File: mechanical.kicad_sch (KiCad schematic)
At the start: 9 parts

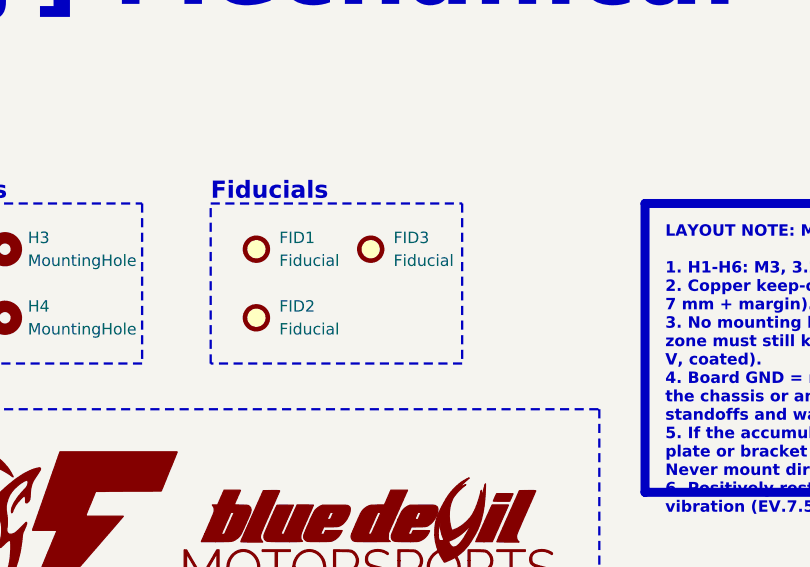
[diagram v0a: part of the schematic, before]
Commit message: PCB&SCH[Fid]: Added 3 fiductals on the back for fab.
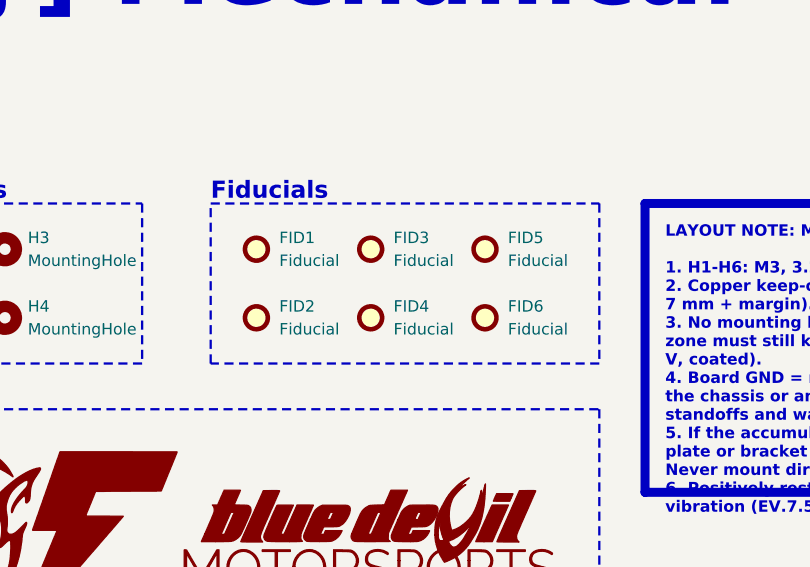
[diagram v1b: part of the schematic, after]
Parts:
- added FID4, FID5, FID6: Fiducial, Fiducial:Fiducial_0.5mm_Mask1mm, symbol Mechanical:Fiducial
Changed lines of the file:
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@@
 	(rectangle
 		(start 147.32 50.8)
-		(end 175.26 68.58)
+		(end 190.5 68.58)
 		(stroke
 			(width 0.254)
@@
 	(symbol
 		(lib_id "Mechanical:Fiducial")
+		(at 165.1 63.5 0)
+		(unit 1)
+		(body_style 1)
+		(exclude_from_sim no)
+		(in_bom no)
+		(on_board yes)
+		(in_pos_files yes)
+		(dnp no)
+		(fields_autoplaced yes)
+		(property "Reference" "FID4"
+			(at 167.64 62.23 0)
+			(show_name no)
+			(do_not_autoplace no)
+			(effects
+				(font
+					(size 1.27 1.27)
+				)
+				(justify left)
+			)
+		)
+		(property "Value" "Fiducial"
+			(at 167.64 64.77 0)
+			(show_name no)
+			(do_not_autoplace no)
+			(effects
+				(font
+					(size 1.27 1.27)
+				)
+				(justify left)
+			)
+		)
+		(property "Footprint" "Fiducial:Fiducial_0.5mm_Mask1mm"
+			(at 165.1 63.5 0)
+			(hide yes)
+			(show_name no)
+			(do_not_autoplace no)
+			(effects
+				(font
+					(size 1.27 1.27)
+				)
+			)
+		)
+		(property "Datasheet" ""
+			(at 165.1 63.5 0)
+			(hide yes)
+			(show_name no)
+			(do_not_autoplace no)
+			(effects
+				(font
+					(size 1.27 1.27)
+				)
+			)
+		)
+		(property "Description" "Fiducial Marker"
+			(at 165.1 63.5 0)
+			(hide yes)
+			(show_name no)
+			(do_not_autoplace no)
+			(effects
+				(font
+					(size 1.27 1.27)
+				)
+			)
+		)
+		(instances
+			(project "bms_slave"
+				(path "/f9e05184-c88b-4a88-ae9c-ab2bdb32be7c/c5103ceb-5325-4a84-a025-9638a412984e/f4a7f626-808e-4d0f-b4d4-b24a2b39d327"
+					(reference "FID4")
+					(unit 1)
+				)
+			)
+		)
+	)
+	(symbol
+		(lib_id "Mechanical:Fiducial")
 		(at 165.1 55.88 0)
 		(unit 1)
@@
 	(symbol
 		(lib_id "Mechanical:Fiducial")
+		(at 177.8 63.5 0)
+		(unit 1)
+		(body_style 1)
+		(exclude_from_sim no)
+		(in_bom no)
+		(on_board yes)
+		(in_pos_files yes)
+		(dnp no)
+		(fields_autoplaced yes)
+		(property "Reference" "FID6"
+			(at 180.34 62.23 0)
+			(show_name no)
+			(do_not_autoplace no)
+			(effects
+				(font
+					(size 1.27 1.27)
+				)
+				(justify left)
+			)
+		)
+		(property "Value" "Fiducial"
+			(at 180.34 64.77 0)
+			(show_name no)
+			(do_not_autoplace no)
+			(effects
+				(font
+					(size 1.27 1.27)
+				)
+				(justify left)
+			)
+		)
+		(property "Footprint" "Fiducial:Fiducial_0.5mm_Mask1mm"
+			(at 177.8 63.5 0)
+			(hide yes)
+			(show_name no)
+			(do_not_autoplace no)
+			(effects
+				(font
+					(size 1.27 1.27)
+				)
+			)
+		)
+		(property "Datasheet" ""
+			(at 177.8 63.5 0)
+			(hide yes)
+			(show_name no)
+			(do_not_autoplace no)
+			(effects
+				(font
+					(size 1.27 1.27)
+				)
+			)
+		)
+		(property "Description" "Fiducial Marker"
+			(at 177.8 63.5 0)
+			(hide yes)
+			(show_name no)
+			(do_not_autoplace no)
+			(effects
+				(font
+					(size 1.27 1.27)
+				)
+			)
+		)
+		(instances
+			(project "bms_slave"
+				(path "/f9e05184-c88b-4a88-ae9c-ab2bdb32be7c/c5103ceb-5325-4a84-a025-9638a412984e/f4a7f626-808e-4d0f-b4d4-b24a2b39d327"
+					(reference "FID6")
+					(unit 1)
+				)
+			)
+		)
+	)
+	(symbol
+		(lib_id "Mechanical:Fiducial")
 		(at 152.4 55.88 0)
 		(unit 1)
@@
 					(unit 1)
 				)
+			)
+		)
+	)
+	(symbol
+		(lib_id "Mechanical:Fiducial")
+		(at 177.8 55.88 0)
+		(unit 1)
+		(body_style 1)
+		(exclude_from_sim no)
+		(in_bom no)
+		(on_board yes)
+		(in_pos_files yes)
+		(dnp no)
+		(fields_autoplaced yes)
+		(property "Reference" "FID5"
+			(at 180.34 54.61 0)
+			(show_name no)
+			(do_not_autoplace no)
+			(effects
+				(font
+					(size 1.27 1.27)
+				)
+				(justify left)
+			)
+		)
+		(property "Value" "Fiducial"
+			(at 180.34 57.15 0)
+			(show_name no)
+			(do_not_autoplace no)
+			(effects
+				(font
+					(size 1.27 1.27)
+				)
+				(justify left)
+			)
+		)
+		(property "Footprint" "Fiducial:Fiducial_0.5mm_Mask1mm"
+			(at 177.8 55.88 0)
+			(hide yes)
+			(show_name no)
+			(do_not_autoplace no)
+			(effects
+				(font
+					(size 1.27 1.27)
+				)
+			)
+		)
+		(property "Datasheet" ""
+			(at 177.8 55.88 0)
+			(hide yes)
+			(show_name no)
+			(do_not_autoplace no)
+			(effects
+				(font
+					(size 1.27 1.27)
+				)
+			)
+		)
+		(property "Description" "Fiducial Marker"
+			(at 177.8 55.88 0)
+			(hide yes)
+			(show_name no)
+			(do_not_autoplace no)
+			(effects
+				(font
+					(size 1.27 1.27)
+				)
+			)
+		)
+		(instances
+			(project "bms_slave"
+				(path "/f9e05184-c88b-4a88-ae9c-ab2bdb32be7c/c5103ceb-5325-4a84-a025-9638a412984e/f4a7f626-808e-4d0f-b4d4-b24a2b39d327"
+					(reference "FID5")
+					(unit 1)
+				)
